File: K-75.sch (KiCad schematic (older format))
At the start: 177 parts, among them J1 Conn_01x04, SW1 SW_Push, U1 ATmega32U4-AU, Y1 Crystal_GND24_Small

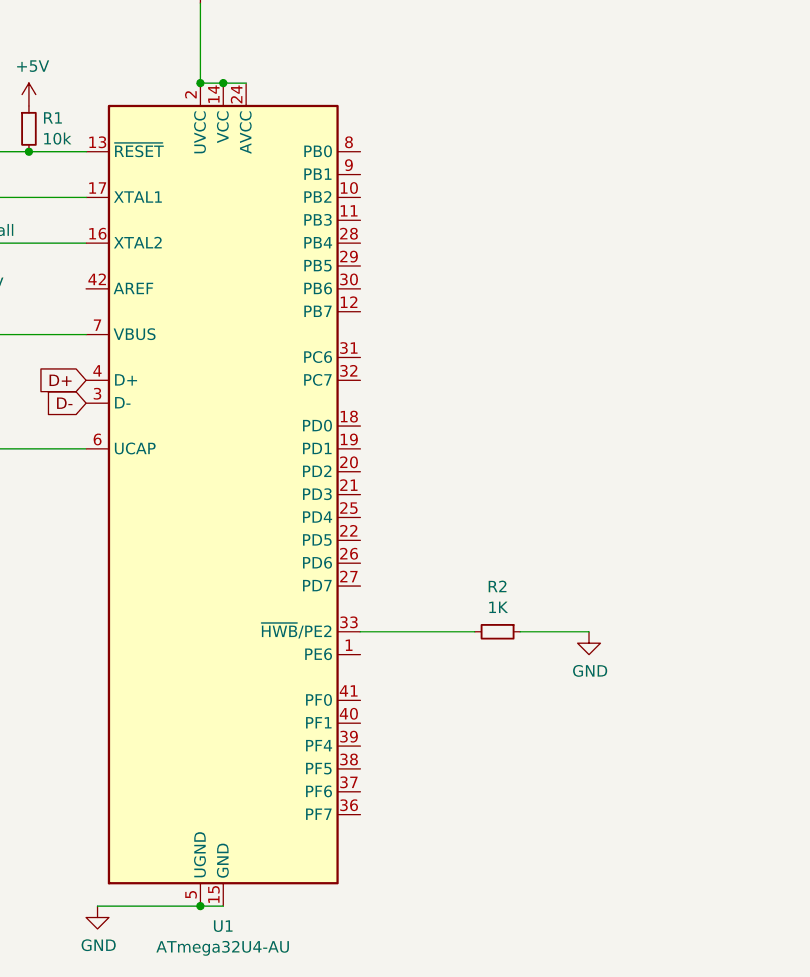
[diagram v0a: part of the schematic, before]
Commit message: Tracing progress
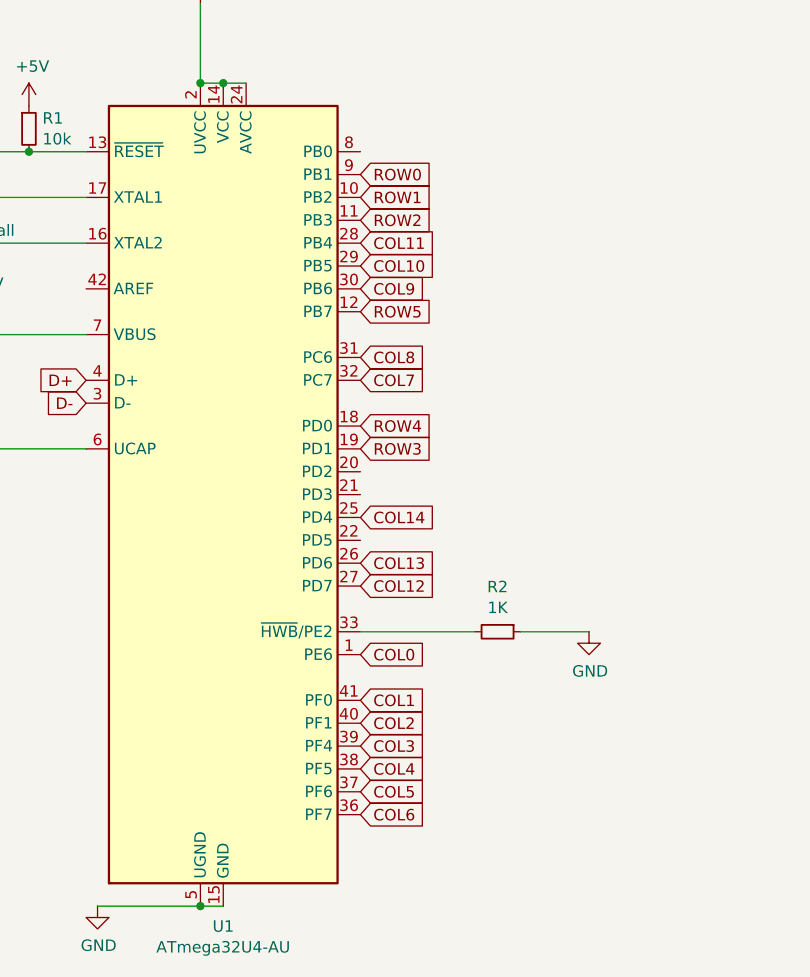
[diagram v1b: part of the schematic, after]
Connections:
- net COL0: now also U1.1 (PE6)
- net COL1: now also U1.41 (PF0)
- net COL10: now also U1.29 (PB5)
- net COL11: now also U1.28 (PB4)
- net COL12: now also U1.27 (PD7)
- net COL13: now also U1.26 (PD6)
- net COL14: now also U1.25 (PD4)
- net COL2: now also U1.40 (PF1)
- net COL3: now also U1.39 (PF4)
- net COL4: now also U1.38 (PF5)
- net COL5: now also U1.37 (PF6)
- net COL6: now also U1.36 (PF7)
- net COL7: now also U1.32 (PC7)
- net COL8: now also U1.31 (PC6)
- net COL9: now also U1.30 (PB6)
- net ROW0: now also U1.9 (PB1)
- net ROW1: now also U1.10 (PB2)
- net ROW2: now also U1.11 (PB3)
- net ROW3: now also U1.19 (PD1)
- net ROW4: now also U1.18 (PD0)
- net ROW5: now also U1.12 (PB7)
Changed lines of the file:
@@
 Connection ~ 10900 3250
 Connection ~ 10900 5000
+Text GLabel 4750 9450 2    50   Input ~ 0
+COL0
+Text GLabel 4750 9650 2    50   Input ~ 0
+COL1
+Text GLabel 4750 9750 2    50   Input ~ 0
+COL2
+Text GLabel 4750 9850 2    50   Input ~ 0
+COL3
+Text GLabel 4750 9950 2    50   Input ~ 0
+COL4
+Text GLabel 4750 10050 2    50   Input ~ 0
+COL5
+Text GLabel 4750 10150 2    50   Input ~ 0
+COL6
+Text GLabel 4750 8250 2    50   Input ~ 0
+COL7
+Text GLabel 4750 8150 2    50   Input ~ 0
+COL8
+Text GLabel 4750 7850 2    50   Input ~ 0
+COL9
+Text GLabel 4750 7750 2    50   Input ~ 0
+COL10
+Text GLabel 4750 7650 2    50   Input ~ 0
+COL11
+Text GLabel 4750 9150 2    50   Input ~ 0
+COL12
+Text GLabel 4750 9050 2    50   Input ~ 0
+COL13
+Text GLabel 4750 8850 2    50   Input ~ 0
+COL14
+Text GLabel 4750 7350 2    50   Input ~ 0
+ROW0
+Text GLabel 4750 7450 2    50   Input ~ 0
+ROW1
+Text GLabel 4750 7550 2    50   Input ~ 0
+ROW2
+Text GLabel 4750 8550 2    50   Input ~ 0
+ROW3
+Text GLabel 4750 8450 2    50   Input ~ 0
+ROW4
+Text GLabel 4750 7950 2    50   Input ~ 0
+ROW5
 $EndSCHEMATC
